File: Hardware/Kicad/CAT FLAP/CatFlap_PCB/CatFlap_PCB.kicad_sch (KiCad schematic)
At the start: 77 parts, among them J1 Conn_01x08, J2 Conn_01x03, J3 ${ALTIUM_VALUE}, J4 Conn_01x03_Socket, J5 Conn_01x03, J6 Conn_01x02, J8 Conn_01x20, J9 Conn_01x20, M1 Motor_DC, Q1 NX3008CBKS, Q2 Q_PMOS_DGS, SW1 SW_Push, SW2 SW_Push, SW3 SW_Push, T1 NX3008NBKS, T2 NX3008NBKS, U1 LM358_DFN, U2 DRV8837DSGR, U3 TPS62132

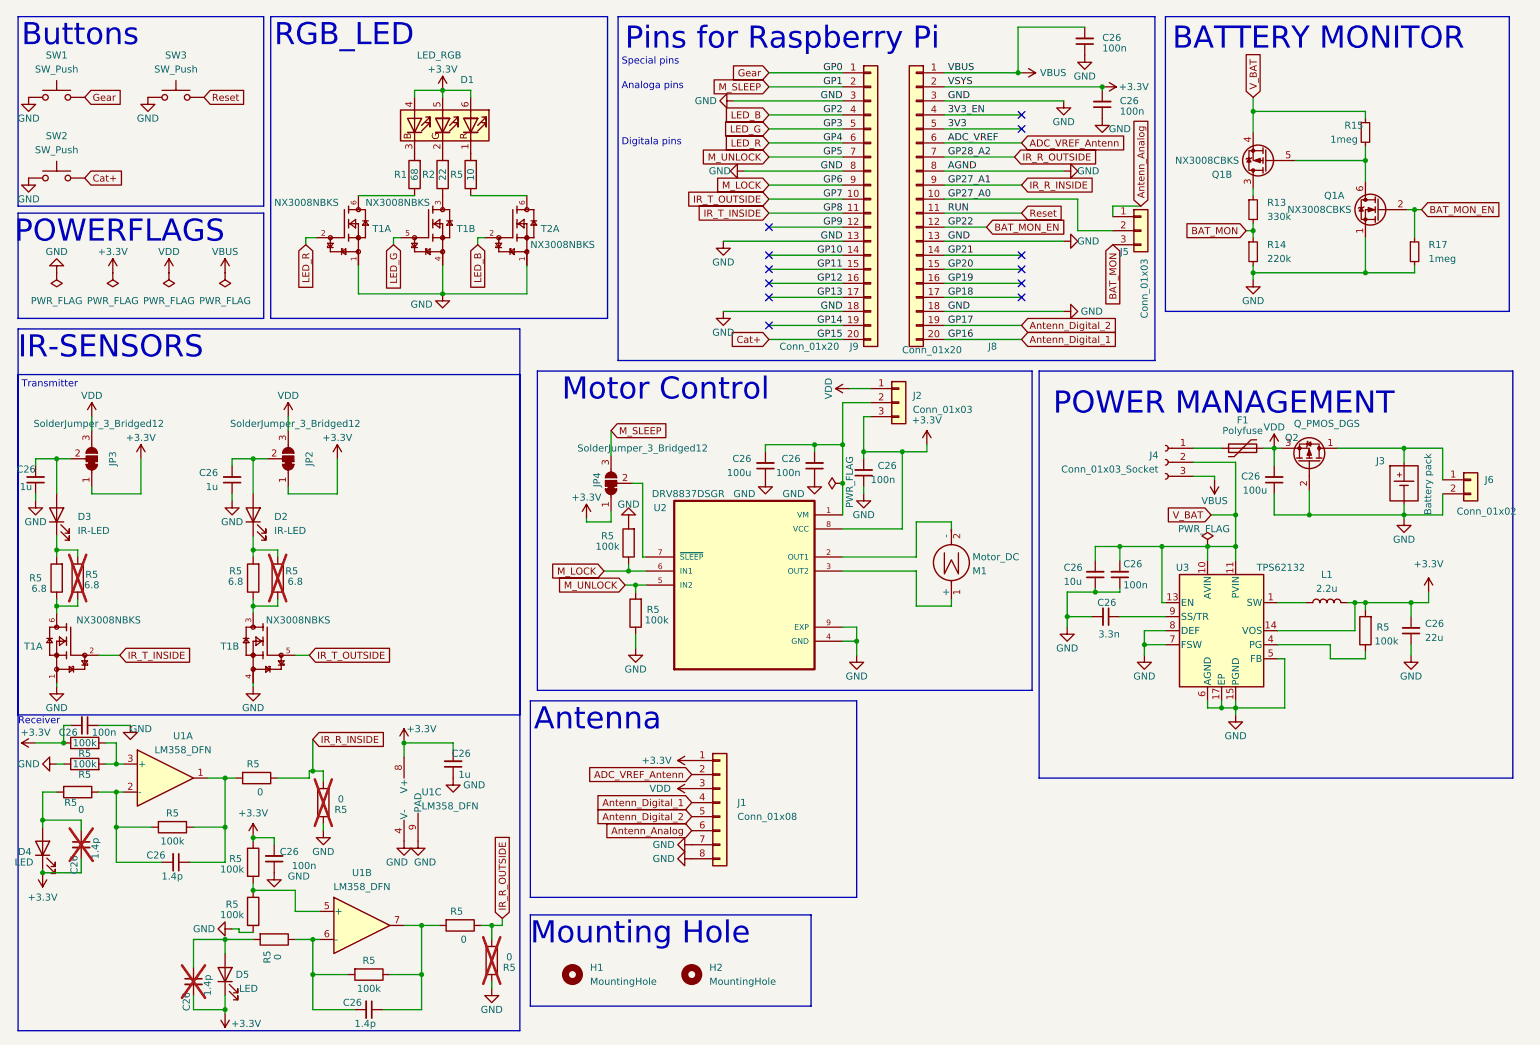
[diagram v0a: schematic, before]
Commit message: Fixed things from first rev of PCB
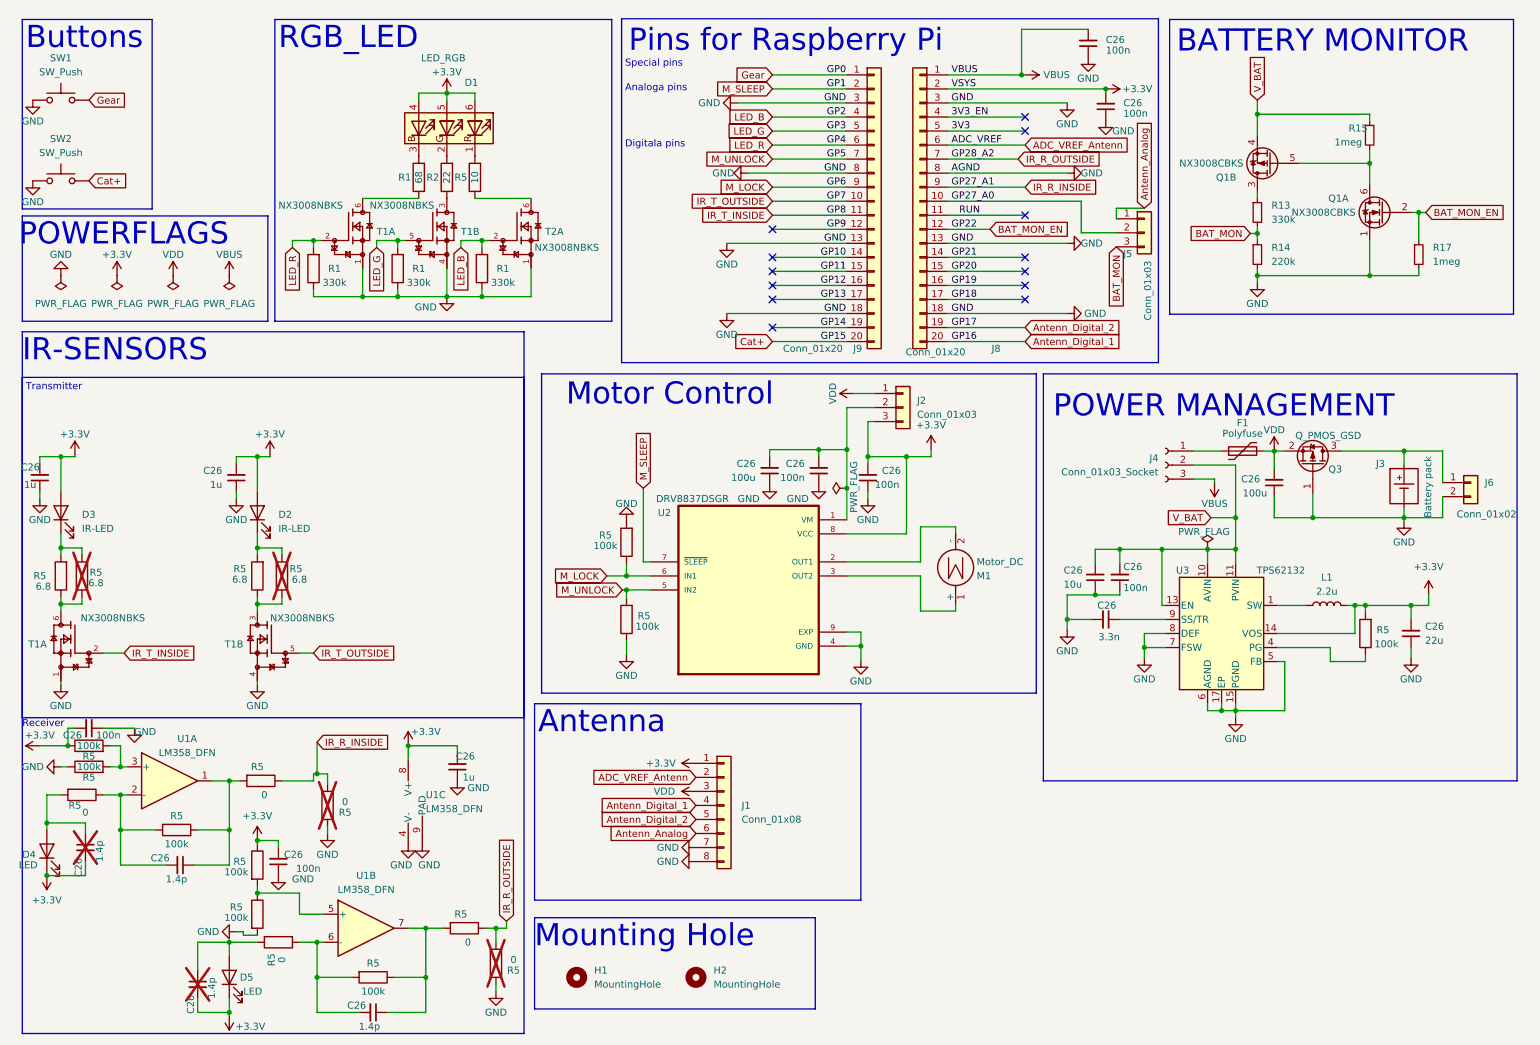
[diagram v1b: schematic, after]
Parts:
- removed JP2, JP3, JP4: SolderJumper_3_Bridged12, Jumper:SolderJumper-3_P1.3mm_Bridged12_RoundedPad1.0x1.5mm, symbol Jumper:SolderJumper_3_Bridged12
- removed Q2: Q_PMOS_DGS, Package_TO_SOT_SMD:SOT-23, symbol Device:Q_PMOS_DGS
- removed SW3: SW_Push, Button_Switch_SMD:SW_Push_1P1T_NO_Vertical_Wuerth_434133025816, symbol Switch:SW_Push
- added Q3: Q_PMOS_GSD, Package_TO_SOT_SMD:SOT-23, symbol Device:Q_PMOS_GSD
- added R1 (x3): 330k, Resistor_SMD:R_0603_1608Metric, symbol Device:R
- Q1: footprint Package_TO_SOT_SMD:TSOT-23-6 -> Package_TO_SOT_SMD:SOT-363_SC-70-6
- SW1, SW2: footprint Button_Switch_THT:SW_PUSH_6mm_H4.3mm -> Button_Switch_SMD:SW_Push_1P1T_NO_CK_KSC6xxJ
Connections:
- net +3.3V: now also C26.2, C26.2, D2.2 (A), D3.2 (A)
- net GND: now also Q3.1 (G), R1.1, R1.1, R1.1
- net LED_B: now also R1.2
- net LED_G: now also R1.2
- net LED_R: now also R1.2
- net M_SLEEP: now also U2.7 (~{SLEEP})
- net VDD: now also Q3.2 (S)
- net at J3.2 (V+), J6.1 (Pin_1): now also Q3.3 (D)
- net Reset renamed RUN
- no-connect marks 12 -> 13
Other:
- moved on the sheet: C26, D1, D2, D3, D4, D5, F1, H1, H2, J1, J2, J3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
